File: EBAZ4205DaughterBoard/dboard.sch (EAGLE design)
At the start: 29 parts, among them IC2 74LS245N, J1 CON-DSUB-15-VGA

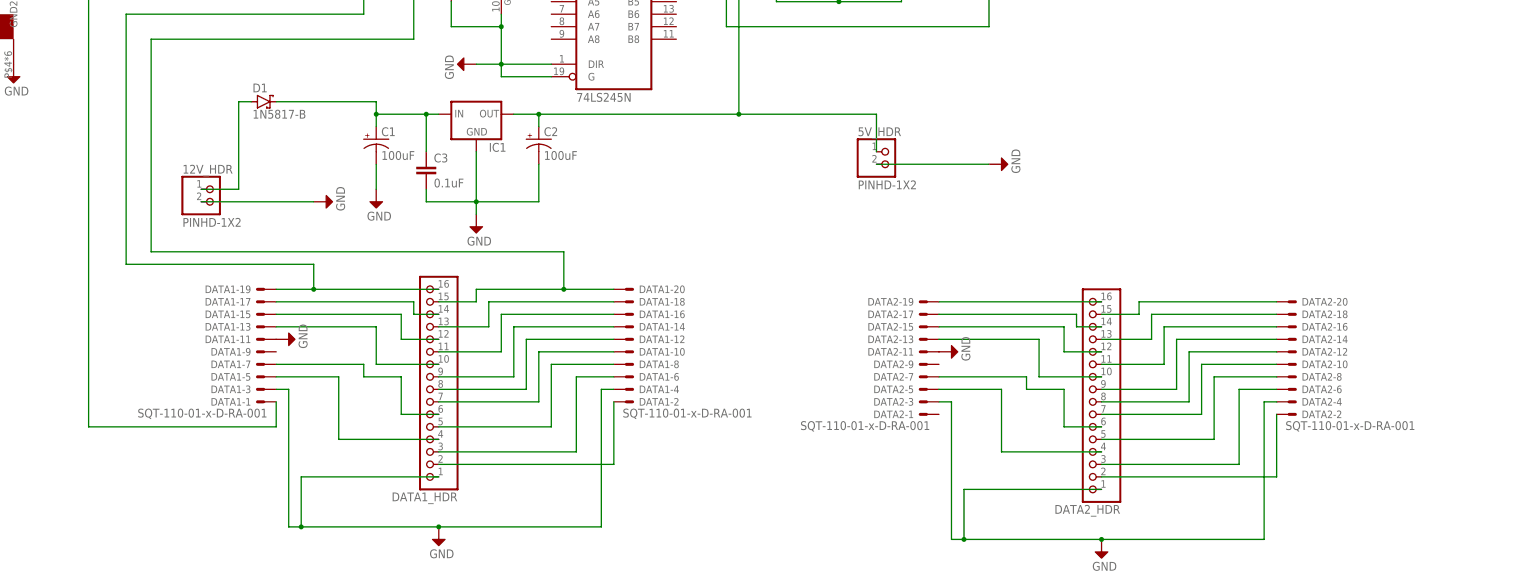
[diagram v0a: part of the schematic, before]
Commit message: Add files via upload
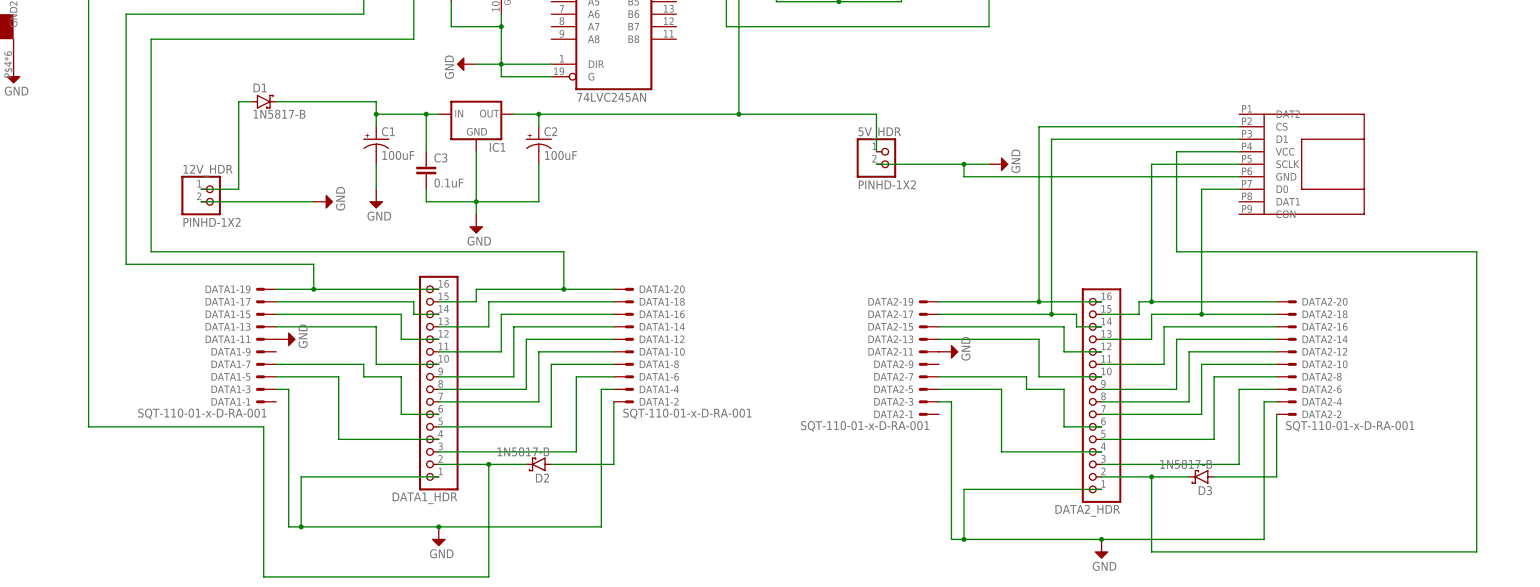
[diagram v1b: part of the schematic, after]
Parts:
- added D2, D3: 1N5817-B, diode:1N5817-B
- added U$2: TF_CARD_BREAKOUT, my-library:OPEN-SMARTTFCARDBREAKOUT
- IC2: value 74LS245N -> 74LVC245AN
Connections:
- removed net DATA1_33V1: DATA1-2.S, DATA1_HDR.2
- removed net G191: DATA1-8.S, DATA1_HDR.5
- removed net G201: DATA1-6.S, DATA1_HDR.3
- removed net J191: DATA1-10.S, DATA1_HDR.7
- removed net K181: DATA1-12.S, DATA1_HDR.8
- removed net KBD+33V: C4.1, DATA1-1.S, IC2P.VCC
- removed net L17: DATA2-19.S, DATA2_HDR.16
- removed net L20: DATA2-17.S, DATA2_HDR.14
- removed net M18: DATA2-18.S, DATA2_HDR.13
- removed net M20: DATA2-20.S, DATA2_HDR.15
- new net DATA1_33V: D2.A, DATA1-2.S
- new net G19: DATA2-8.S, DATA2_HDR.5
- new net G20: DATA2-6.S, DATA2_HDR.3
- new net J19: DATA2-10.S, DATA2_HDR.7
- new net K18: DATA2-12.S, DATA2_HDR.8
- new net KBD_VCC: C4.1, D2.C, DATA1_HDR.2, IC2P.VCC
- new net SD_CS: DATA2-19.S, DATA2_HDR.16, U$2.CS
- new net SD_MISO: DATA2-18.S, DATA2_HDR.13, U$2.D0
- new net SD_MOSI: DATA2-17.S, DATA2_HDR.14, U$2.D1
- new net SD_SCLK: DATA2-20.S, DATA2_HDR.15, U$2.SCLK
- new net SD_VCC: D3.C, DATA2_HDR.2, U$2.VCC
- net A20: now also DATA1-6.S, DATA1_HDR.3; no longer DATA2-6.S, DATA2_HDR.3
- net B19: now also DATA1-8.S, DATA1_HDR.5; no longer DATA2-8.S, DATA2_HDR.5
- net C20: now also DATA1-10.S, DATA1_HDR.7; no longer DATA2-10.S, DATA2_HDR.7
- net DATA2_33V: now also D3.A; no longer DATA2_HDR.2
- net GND: now also U$2.GND
- net H17: now also DATA1-12.S, DATA1_HDR.8; no longer DATA2-12.S, DATA2_HDR.8
